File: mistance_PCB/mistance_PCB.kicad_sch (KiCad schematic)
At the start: 44 parts, among them J1 USB_B_Micro, J2 USB_B_Micro, J3 GRPB052VWVN-RC, Q1 Q_PMOS_DSG, U1 ESP32-WROOM-32E, U2 TPS61200DRC, U3 MCP73831-2-OT, U4 AMS1117-3.3, U5 CP2104, U6 TPS3839DBZ

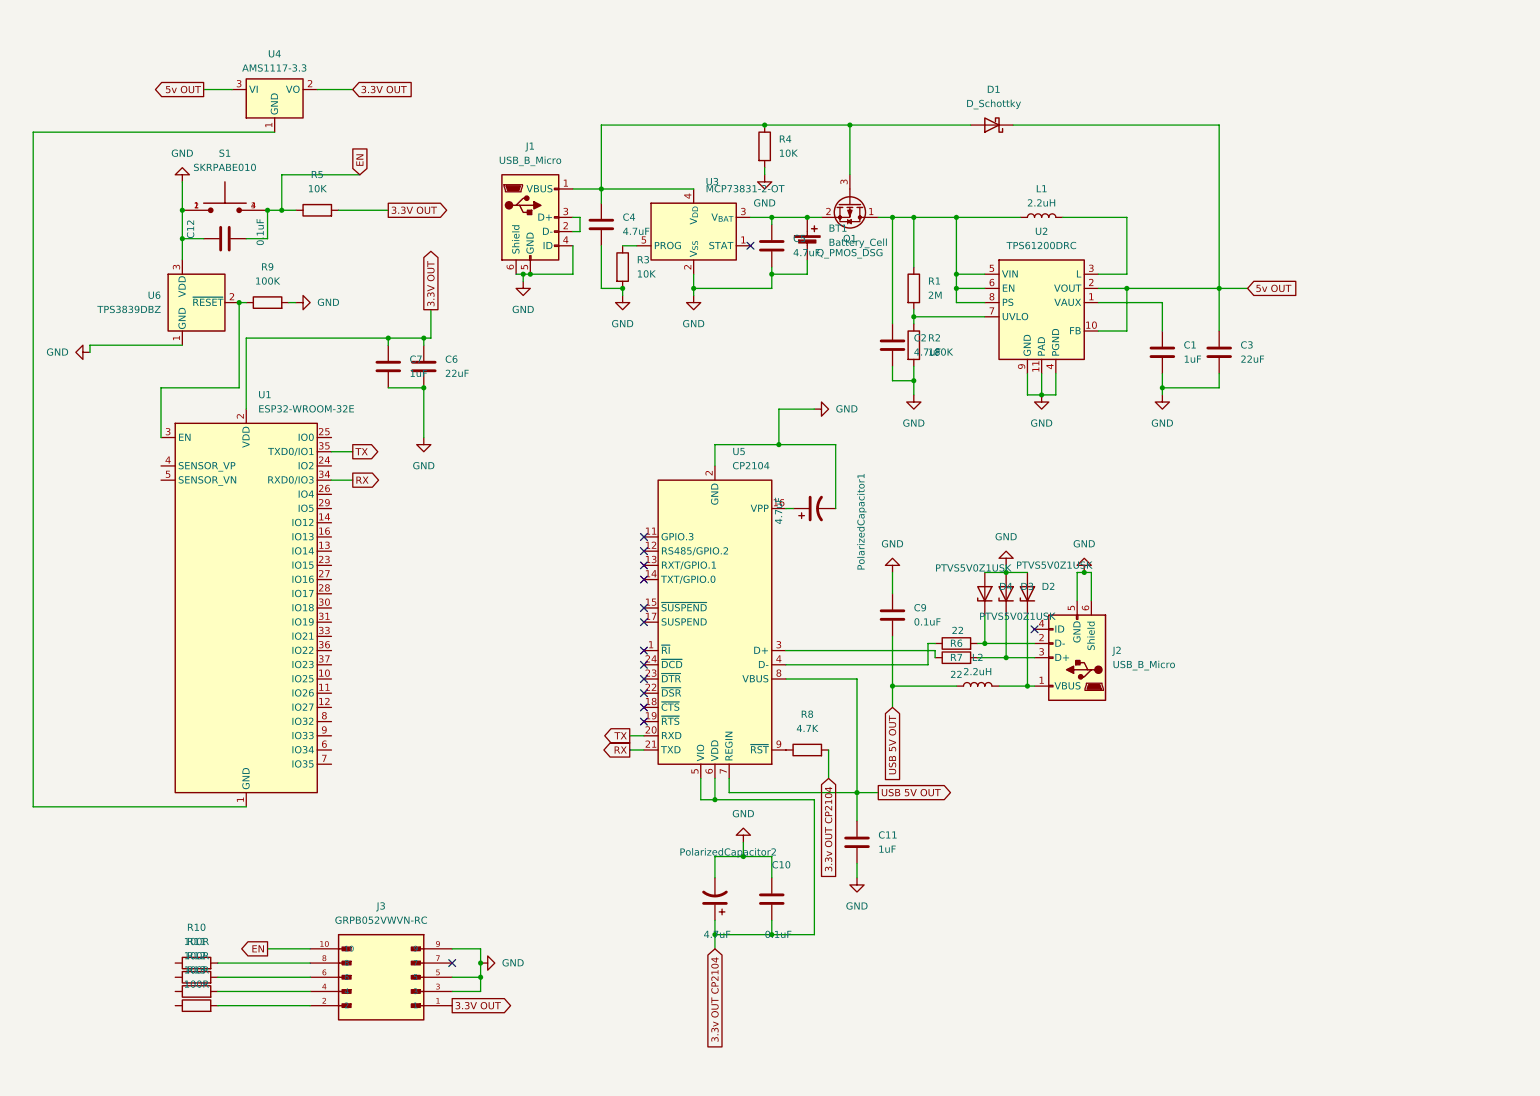
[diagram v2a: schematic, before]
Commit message: PCB update
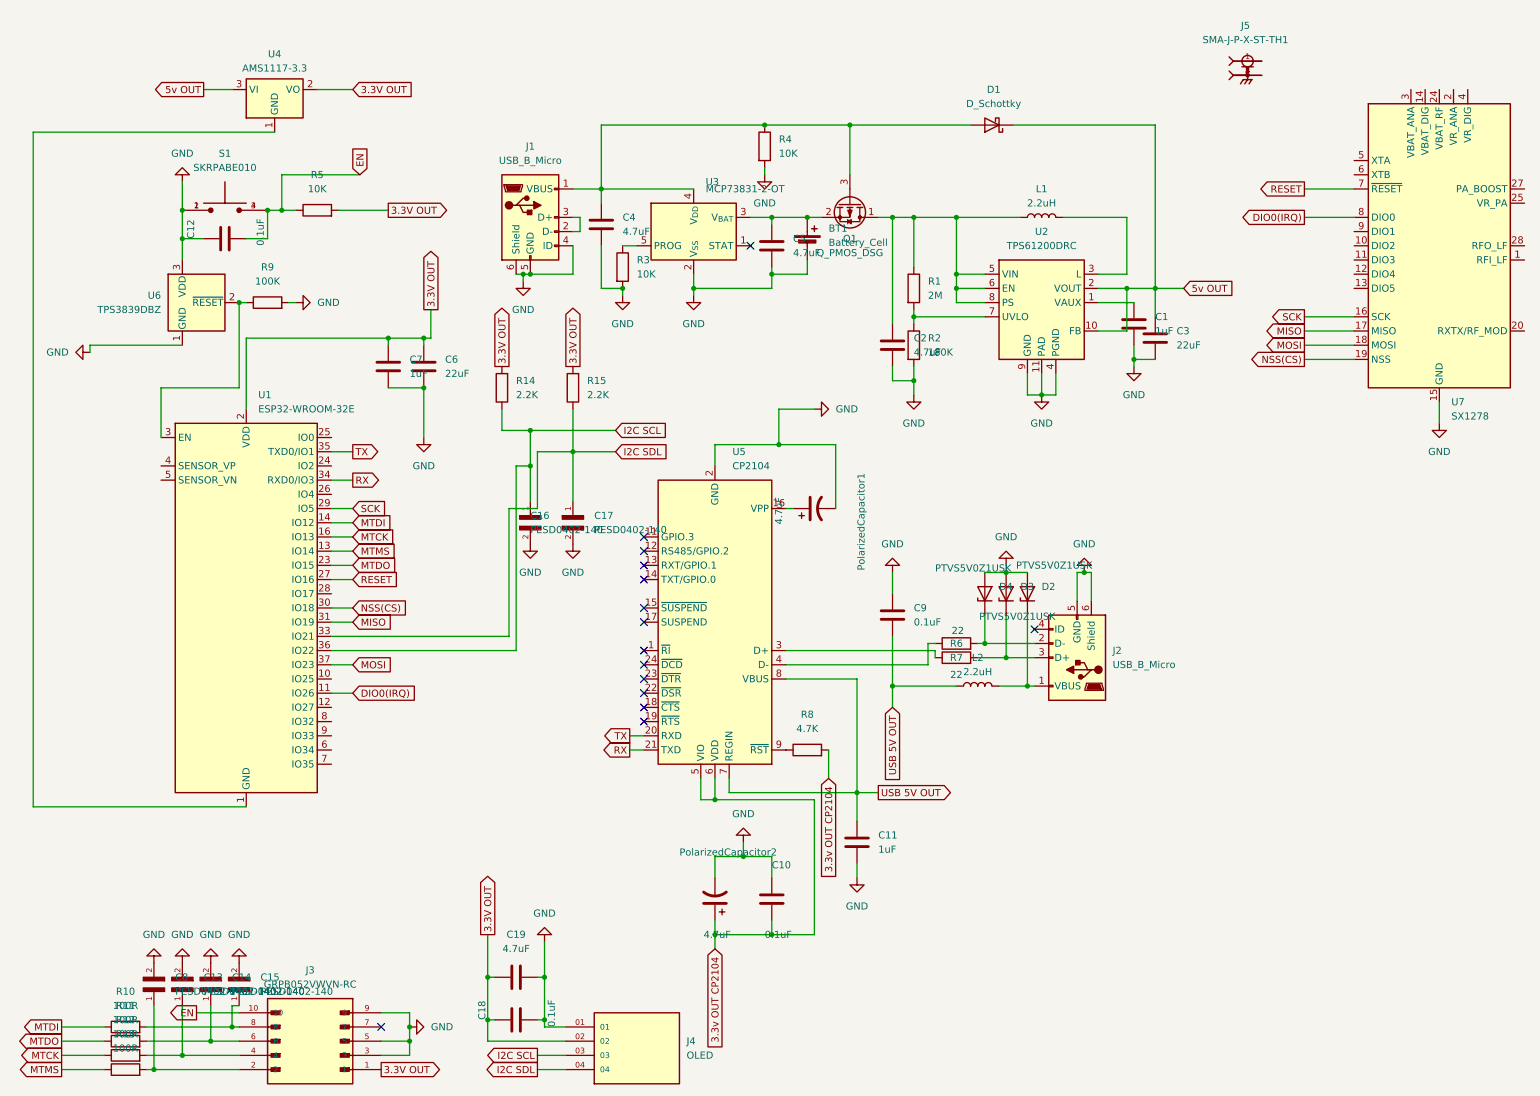
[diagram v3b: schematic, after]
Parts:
- added C13, C14, C15, C16, C17, C8: PESD0402-140, PESD0402-140:RESC1005X35N, symbol PESD0402-140:PESD0402-140
- added C18: 0.1uF, Capacitor_SMD:C_1210_3225Metric, symbol Device:C
- added C19: 4.7uF, Capacitor_SMD:C_1210_3225Metric, symbol Device:C
- added J4: OLED, HTSW-104-20-TM-S:SAMTEC_HTSW-104-20-TM-S, symbol HTSW-104-20-TM-S:HTSW-104-20-TM-S
- added J5: SMA-J-P-X-ST-TH1, SMA-J-P-X-ST-TH1:SAMTEC_SMA-J-P-X-ST-TH1, symbol SMA-J-P-X-ST-TH1:SMA-J-P-X-ST-TH1
- added R14, R15: 2.2K, Resistor_SMD:R_0603_1608Metric, symbol Device:R
- added U7: SX1278, Package_DFN_QFN:QFN-28-1EP_6x6mm_P0.65mm_EP4.8x4.8mm, symbol RF:SX1278
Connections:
- net 3.3V OUT: now also C18.1, C19.1, J4.02, R14.2, R15.2
- net GND: now also C13.2, C14.2, C15.2, C16.2, C17.2, C18.2, C19.2, C8.2, J4.01, U7.15 (GND), U7.21 (GND), U7.22 (GND), U7.23 (GND), U7.26 (GND), U7.29 (GND)
- net MTDI: now reaches R10.1
- net MTDI: now also U1.14 (IO12)
- net at J3.8, R10.2: now also C15.1
- net MTDO: now reaches R11.1
- net MTDO: now also U1.23 (IO15)
- net at J3.6, R11.2: now also C14.1
- net MTMS: now reaches R13.1
- net MTMS: now also U1.13 (IO14)
- net at J3.2, R13.2: now also C8.1
- net MTCK: now reaches R12.1
- net MTCK: now also U1.16 (IO13)
- net at J3.4, R12.2: now also C13.1
- net DIO0(IRQ): now reaches U1.11 (IO26)
- net DIO0(IRQ): now also U7.8 (DIO0)
- net RESET: now reaches U1.27 (IO16)
- net RESET: now also U7.7 (~{RESET})
- net SCK: now reaches U1.29 (IO5)
- net SCK: now also U7.16 (SCK)
- net NSS(CS): now reaches U1.30 (IO18)
- net NSS(CS): now also U7.19 (NSS)
- net MISO: now reaches U1.31 (IO19)
- net MISO: now also U7.17 (MISO)
- net I2C SDL: now reaches U1.33 (IO21)
- net I2C SDL: now also C17.1, J4.04, R15.1
- net I2C SCL: now reaches U1.36 (IO22)
- net I2C SCL: now also C16.1, J4.03, R14.1
- net MOSI: now reaches U1.37 (IO23)
- net MOSI: now also U7.18 (MOSI)
- new net: J5.2, J5.3, J5.4, J5.5
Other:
- moved on the sheet: C1, C3, J3, R10, R11, R12, R13

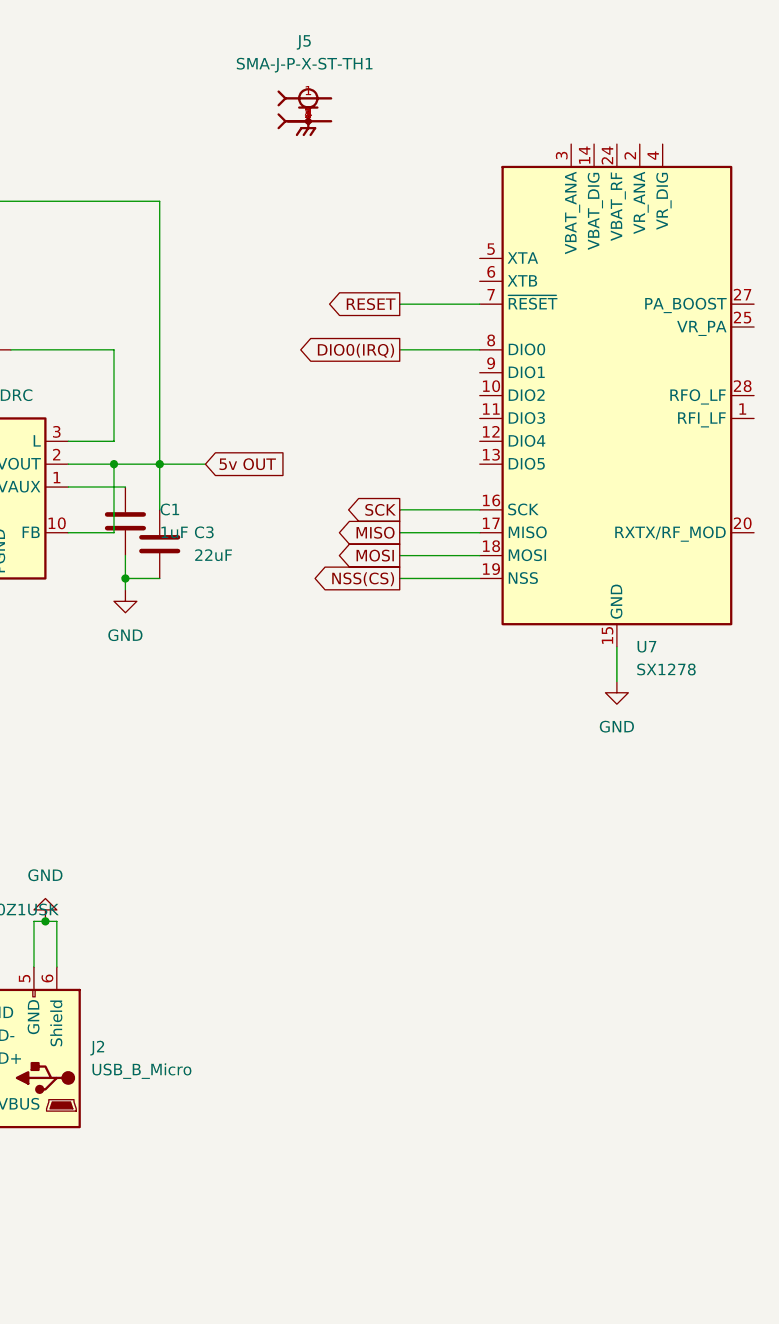
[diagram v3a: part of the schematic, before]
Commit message: PCB update
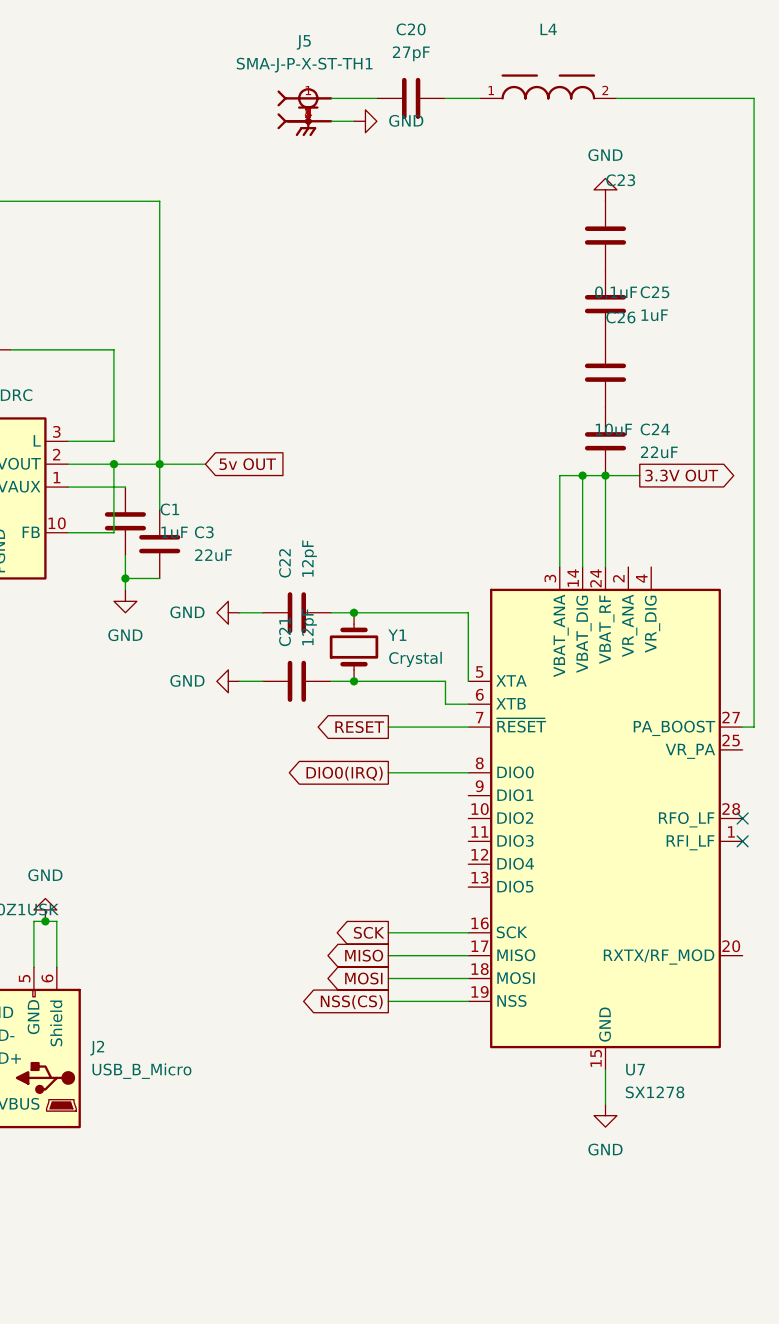
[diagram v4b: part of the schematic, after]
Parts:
- added C20: 27pF, Capacitor_SMD:C_0603_1608Metric, symbol Device:C
- added C21, C22: 12pF, Capacitor_SMD:C_0402_1005Metric, symbol Device:C
- added C23: 0.1uF, Capacitor_SMD:C_1210_3225Metric, symbol Device:C
- added C24: 22uF, Capacitor_SMD:C_1210_3225Metric, symbol Device:C
- added C25: 1uF, Capacitor_SMD:C_1210_3225Metric, symbol Device:C
- added C26: 10uF, Capacitor_SMD:C_1210_3225Metric, symbol Device:C
- added L4: WE-TPC_2811, WE-TPC_2811:WE-TPC_2811, symbol WE-TPC_2811:WE-TPC_2811
- added Y1: Crystal, Crystal:Crystal_SMD_2012-2Pin_2.0x1.2mm, symbol Device:Crystal
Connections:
- net 3.3V OUT: now also U7.14 (VBAT_DIG), U7.24 (VBAT_RF), U7.3 (VBAT_ANA), C24.2
- net GND: now also J5.2, J5.3, J5.4, J5.5, C21.1, C22.1, C23.1
- net at U7.27 (PA_BOOST): now also L4.2
- net at U7.5 (XTA): now also C22.2, Y1.2
- net at U7.6 (XTB): now also C21.2, Y1.1
- net at J5.1: now also C20.1
- new net: C20.2, L4.1
- new net: C23.2, C25.1
- new net: C25.2, C26.1
- new net: C24.1, C26.2
- no-connect marks 15 -> 17
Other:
- moved on the sheet: U7

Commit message: PCB update
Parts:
- S1: footprint SKRPABE010:SW_SKRPABE010 -> Diode_SMD:SW_SKRPABE010
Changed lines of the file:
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@@
 			)
 		)
-		(property "Footprint" "SKRPABE010:SW_SKRPABE010"
+		(property "Footprint" "Diode_SMD:SW_SKRPABE010"
 			(at 49.53 40.64 0)
 			(effects

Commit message: PCB first chack end
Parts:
- U1: footprint RF_Module:ESP32-WROOM-32D -> RF_Module:ESP32-WROOM-32E
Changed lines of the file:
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@@
 	(wire
 		(pts
+			(xy 161.29 25.4) (xy 182.88 25.4)
+		)
+		(stroke
+			(width 0)
+			(type default)
+		)
+	)
+	(wire
+		(pts
 			(xy 111.76 41.91) (xy 113.03 41.91)
 		)
@@
 	(wire
 		(pts
-			(xy 161.29 25.4) (xy 182.88 25.4)
-		)
-		(stroke
-			(width 0)
-			(type default)
-		)
-	)
-	(wire
-		(pts
 			(xy 176.53 120.65) (xy 176.53 119.38)
 		)
@@
 			)
 		)
-		(property "Footprint" "RF_Module:ESP32-WROOM-32D"
+		(property "Footprint" "RF_Module:ESP32-WROOM-32E"
 			(at 69.85 146.05 0)
 			(effects
